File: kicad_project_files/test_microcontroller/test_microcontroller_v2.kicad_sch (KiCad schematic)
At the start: 40 parts, among them J1 USB_C_Receptacle_USB2.0, SW1 SW_Push, SW2 SW_Push, SW3 SW_Push, SW4 SW_Push, SW5 SW_Push, SW6 SW_Push, SW7 SW_Push, SW8 SW_Push, SW9 SW_Push, U1 ATmega32U4-A, Y1 16mhz

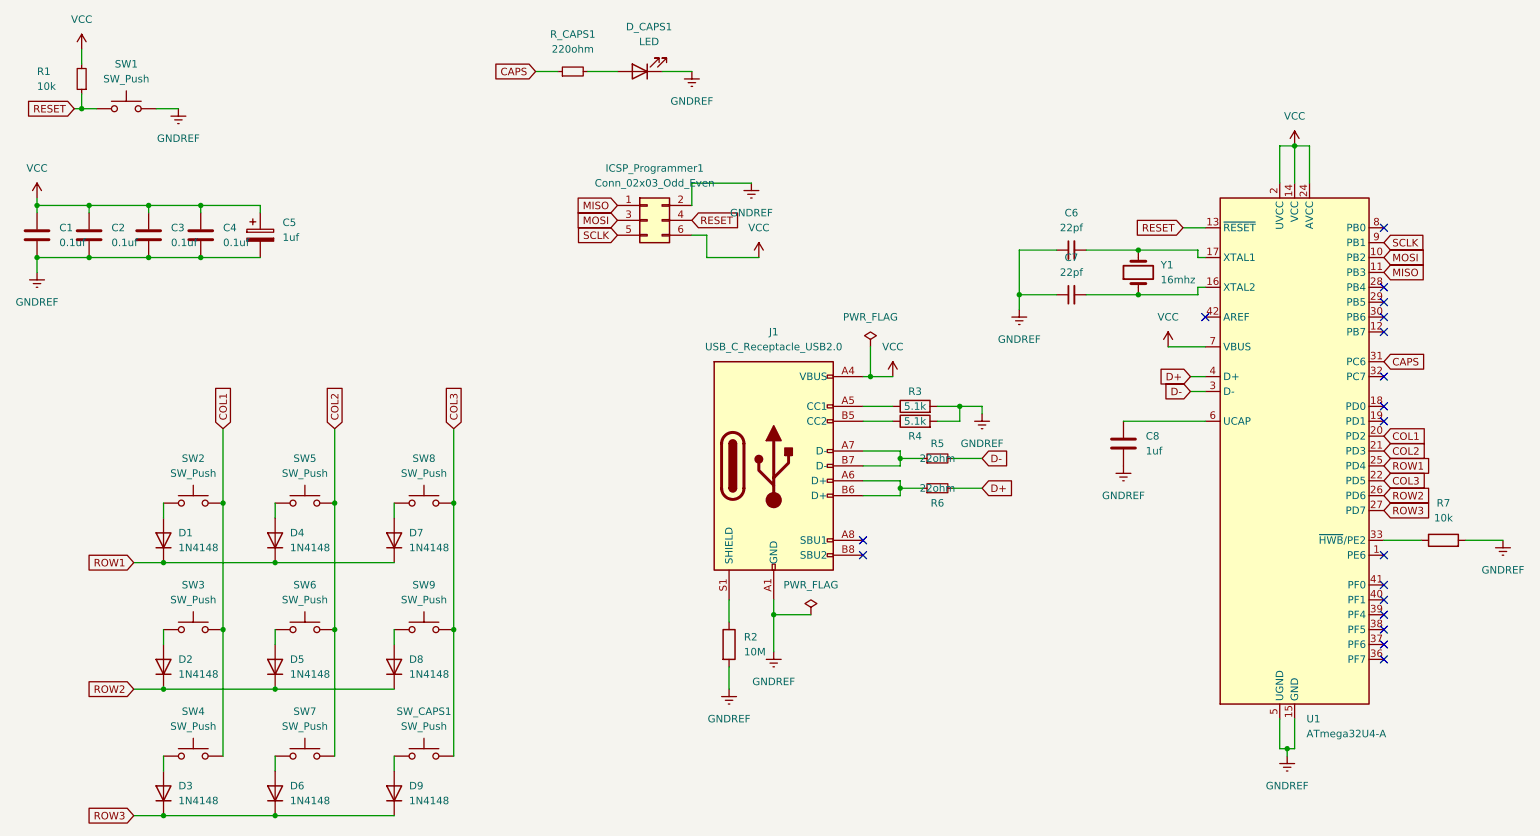
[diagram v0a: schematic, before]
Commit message: Revert "add diode to pcb"
This reverts commit 20722a3885263840da117607ee800e449ae5a56b.
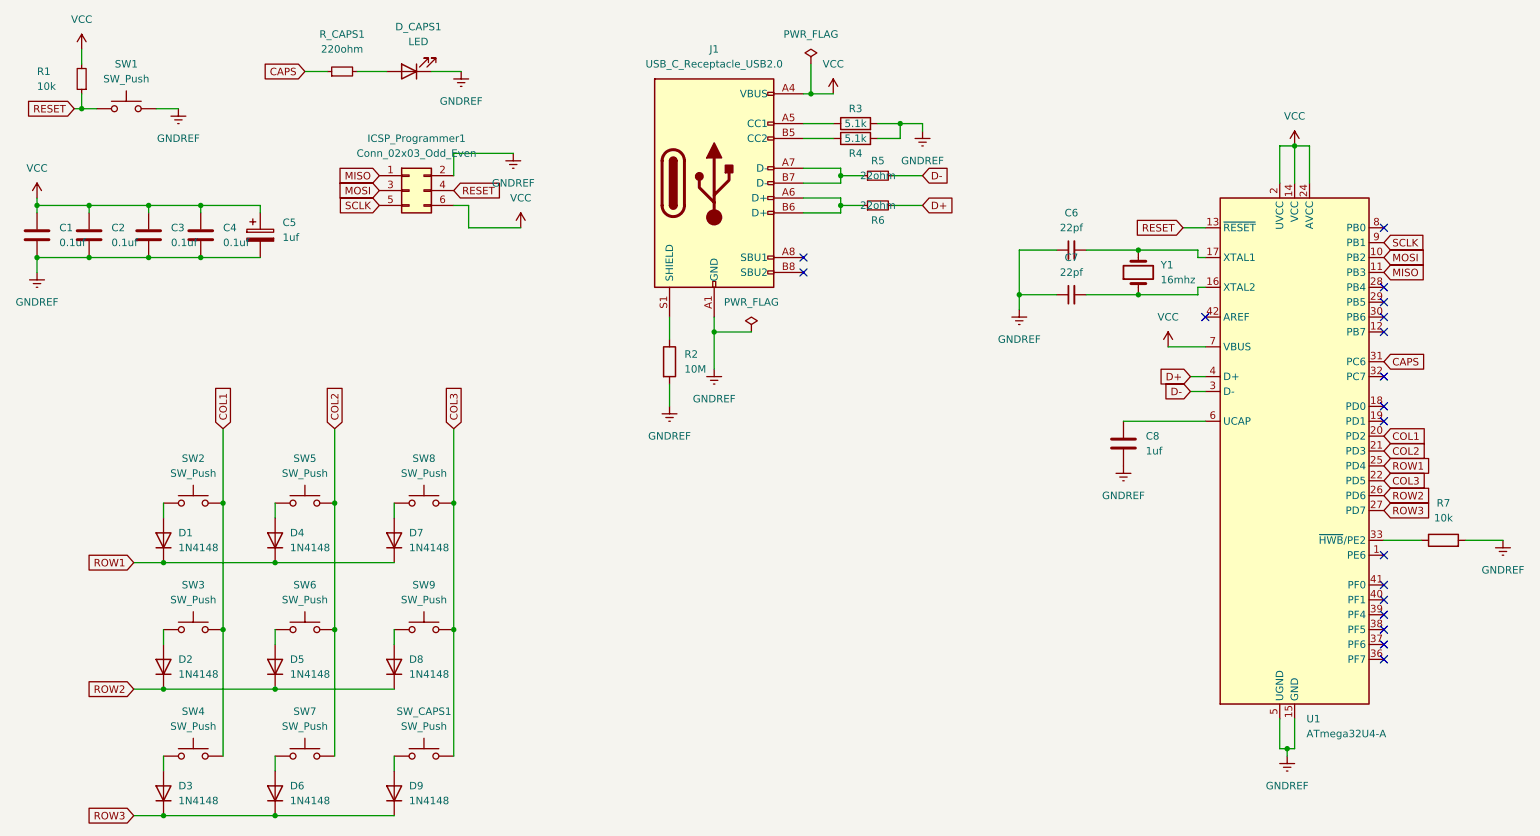
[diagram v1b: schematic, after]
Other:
- moved on the sheet: D_CAPS1, ICSP_Programmer1, J1, R2, R3, R4, R5, R6, R_CAPS1
